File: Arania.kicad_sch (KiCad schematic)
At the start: 13 parts, among them J13 LASER, J14 GP03, J15 GP04, J16 GP04, J17 GP04, J18 GP04, J19 GP04, J20 GP04, J21 GP04, J22 GP04, J23 GP04, Q1 MMBT3904

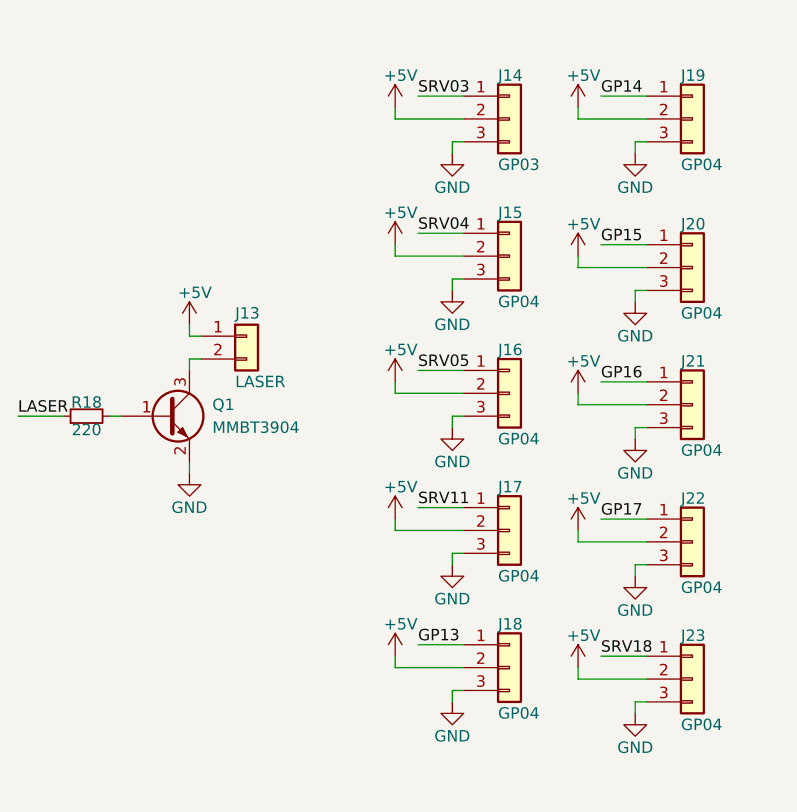
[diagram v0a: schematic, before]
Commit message: Finalizo el esquematico
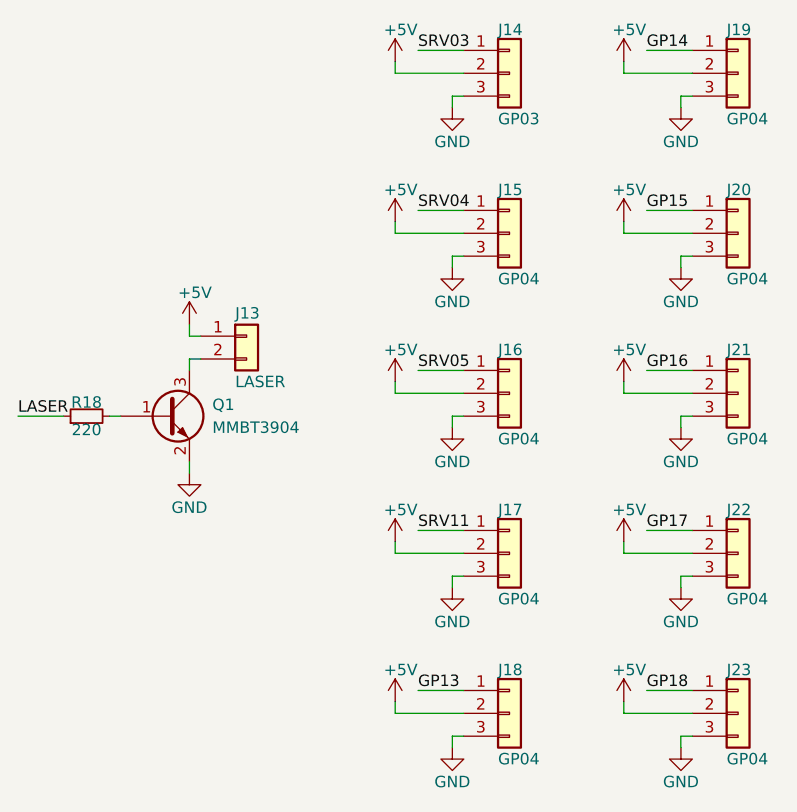
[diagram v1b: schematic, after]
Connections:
- net SRV18 renamed GP18
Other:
- moved on the sheet: J14, J15, J17, J18, J19, J20, J21, J22, J23
